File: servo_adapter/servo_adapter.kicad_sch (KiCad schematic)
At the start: 20 parts, among them J1 T4140012081-000, J2 Conn_01x10_Socket, J3 Conn_01x02_Socket, J4 T4141012051-000, U1 MUN5233T1G, U2 MUN5233T1G, U3 MUN5233T1G, U4 MUN5233T1G

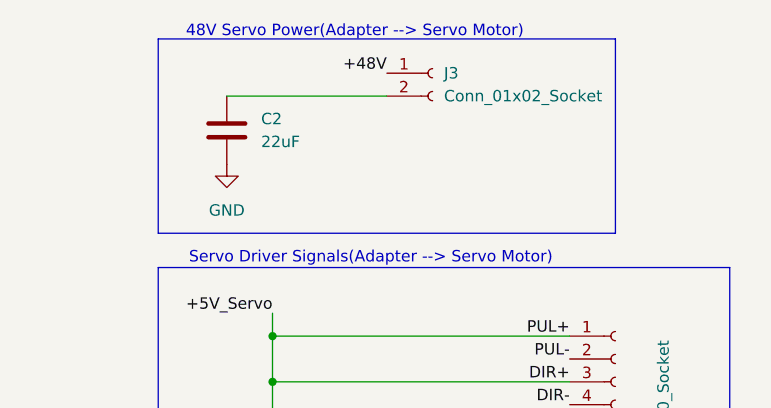
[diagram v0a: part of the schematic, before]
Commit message: Added the 2pin power connector to servo adapter board and schematic.
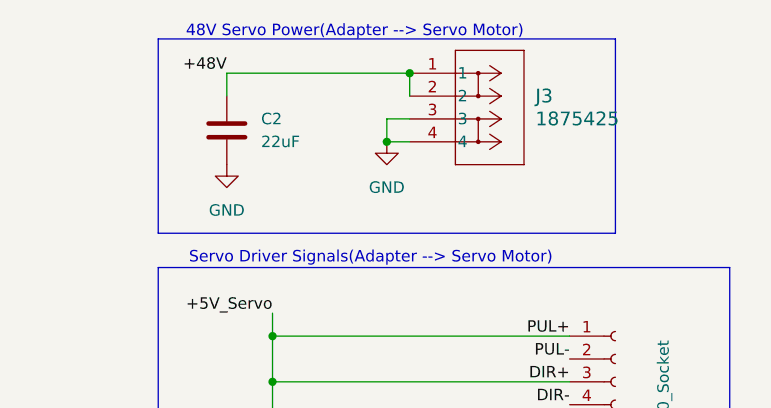
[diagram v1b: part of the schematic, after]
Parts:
- removed J3: Conn_01x02_Socket, Connector_Phoenix_MC:PhoenixContact_MCV_1,5_2-GF-3.81_1x02_P3.81mm_Vertical_ThreadedFlange_MountHole, symbol Connector:Conn_01x02_Socket
- added J3: 1875425, servo_adapter_fp:CONN_1875425, symbol 1875425:1875425
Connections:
- net +48V: now also C2.1, J3.1, J3.2
- net GND: now also J3.3, J3.4
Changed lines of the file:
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@@
 	)
 	(junction
+		(at 241.3 29.21)
+		(diameter 0)
+		(color 0 0 0 0)
+	)
+	(junction
 		(at 241.3 86.36)
 		(diameter 0)
@@
 	)
 	(junction
+		(at 243.84 21.59)
+		(diameter 0)
+		(color 0 0 0 0)
+	)
+	(junction
 		(at 33.02 38.1)
 		(diameter 0)
@@
 	(wire
 		(pts
+			(xy 223.52 21.59) (xy 223.52 24.13)
+		)
+		(stroke
+			(width 0)
+			(type default)
+		)
+	)
+	(wire
+		(pts
 			(xy 228.6 50.8) (xy 228.6 48.26)
 		)
@@
 	(wire
 		(pts
+			(xy 241.3 26.67) (xy 241.3 29.21)
+		)
+		(stroke
+			(width 0)
+			(type default)
+		)
+	)
+	(wire
+		(pts
 			(xy 81.28 165.1) (xy 81.28 170.18)
 		)
@@
 	(wire
 		(pts
+			(xy 243.84 29.21) (xy 241.3 29.21)
+		)
+		(stroke
+			(width 0)
+			(type default)
+		)
+	)
+	(wire
+		(pts
 			(xy 228.6 78.74) (xy 228.6 86.36)
 		)
@@
 	(wire
 		(pts
+			(xy 223.52 21.59) (xy 243.84 21.59)
+		)
+		(stroke
+			(width 0)
+			(type default)
+		)
+	)
+	(wire
+		(pts
+			(xy 243.84 26.67) (xy 241.3 26.67)
+		)
+		(stroke
+			(width 0)
+			(type default)
+		)
+	)
+	(wire
+		(pts
 			(xy 25.4 30.48) (xy 38.1 30.48)
 		)
@@
 	(wire
 		(pts
-			(xy 38.1 35.56) (xy 33.02 35.56)
+			(xy 243.84 21.59) (xy 243.84 24.13)
 		)
 		(stroke
@@
 	(wire
 		(pts
-			(xy 261.62 71.12) (xy 228.6 71.12)
+			(xy 38.1 35.56) (xy 33.02 35.56)
 		)
 		(stroke
@@
 	(wire
 		(pts
-			(xy 38.1 38.1) (xy 33.02 38.1)
+			(xy 261.62 71.12) (xy 228.6 71.12)
 		)
 		(stroke
@@
 	(wire
 		(pts
-			(xy 30.48 78.74) (xy 46.99 78.74)
+			(xy 38.1 38.1) (xy 33.02 38.1)
 		)
 		(stroke
@@
 	(wire
 		(pts
-			(xy 223.52 24.13) (xy 241.3 24.13)
+			(xy 30.48 78.74) (xy 46.99 78.74)
 		)
 		(stroke
@@
 	)
 	(label "+48V"
-		(at 241.3 21.59 180)
+		(at 223.52 21.59 180)
 		(effects
 			(font
@@
 	)
 	(symbol
+		(lib_id "power:GND")
+		(at 241.3 29.21 0)
+		(unit 1)
+		(exclude_from_sim no)
+		(in_bom yes)
+		(on_board yes)
+		(dnp no)
+		(fields_autoplaced yes)
+		(property "Reference" "#PWR011"
+			(at 241.3 35.56 0)
+			(effects
+				(font
+					(size 1.27 1.27)
+				)
+				(hide yes)
+			)
+		)
+		(property "Value" "GND"
+			(at 241.3 34.29 0)
+			(effects
+				(font
+					(size 1.27 1.27)
+				)
+			)
+		)
+		(property "Footprint" ""
+			(at 241.3 29.21 0)
+			(effects
+				(font
+					(size 1.27 1.27)
+				)
+				(hide yes)
+			)
+		)
+		(property "Datasheet" ""
+			(at 241.3 29.21 0)
+			(effects
+				(font
+					(size 1.27 1.27)
+				)
+				(hide yes)
+			)
+		)
+		(property "Description" "Power symbol creates a global label with name \"GND\" , ground"
+			(at 241.3 29.21 0)
+			(effects
+				(font
+					(size 1.27 1.27)
+				)
+				(hide yes)
+			)
+		)
+		(pin "1"
+		)
+		(instances
+			(project "servo_adapter"
+				(path "/d2a6932a-1682-4170-bbbb-2fb2c0f935d7"
+					(reference "#PWR011")
+					(unit 1)
+				)
+			)
+		)
+	)
+	(symbol
 		(lib_id "Device:C")
 		(at 223.52 27.94 0)
@@
 	)
 	(symbol
-		(lib_id "Connector:Conn_01x02_Socket")
-		(at 246.38 21.59 0)
-		(unit 1)
-		(exclude_from_sim no)
-		(in_bom yes)
-		(on_board yes)
-		(dnp no)
-		(fields_autoplaced yes)
-		(property "Reference" "J3"
-			(at 247.65 21.5899 0)
-			(effects
-				(font
-					(size 1.27 1.27)
-				)
-				(justify left)
-			)
-		)
-		(property "Value" "Conn_01x02_Socket"
-			(at 247.65 24.1299 0)
-			(effects
-				(font
-					(size 1.27 1.27)
-				)
-				(justify left)
-			)
-		)
-		(property "Footprint" "Connector_Phoenix_MC:PhoenixContact_MCV_1,5_2-GF-3.81_1x02_P3.81mm_Vertical_ThreadedFlange_MountHole"
-			(at 246.38 21.59 0)
-			(effects
-				(font
-					(size 1.27 1.27)
-				)
-				(hide yes)
-			)
-		)
-		(property "Datasheet" "~"
-			(at 246.38 21.59 0)
-			(effects
-				(font
-					(size 1.27 1.27)
-				)
-				(hide yes)
-			)
-		)
-		(property "Description" "Generic connector, single row, 01x02, script generated"
-			(at 246.38 21.59 0)
-			(effects
-				(font
-					(size 1.27 1.27)
-				)
-				(hide yes)
-			)
-		)
-		(pin "2"
-		)
-		(pin "1"
-		)
-		(instances
-			(project ""
-				(path "/d2a6932a-1682-4170-bbbb-2fb2c0f935d7"
-					(reference "J3")
-					(unit 1)
-				)
-			)
-		)
-	)
-	(symbol
 		(lib_id "power:PWR_FLAG")
 		(at 54.61 72.39 180)
@@
 					(unit 1)
 				)
+			)
+		)
+	)
+	(symbol
+		(lib_id "1875425:1875425")
+		(at 243.84 21.59 0)
+		(unit 1)
+		(exclude_from_sim no)
+		(in_bom yes)
+		(on_board yes)
+		(dnp no)
+		(fields_autoplaced yes)
+		(property "Reference" "J3"
+			(at 257.81 24.1299 0)
+			(effects
+				(font
+					(size 1.524 1.524)
+				)
+				(justify left)
+			)
+		)
+		(property "Value" "1875425"
+			(at 257.81 26.6699 0)
+			(effects
+				(font
+					(size 1.524 1.524)
+				)
+				(justify left)
+			)
+		)
+		(property "Footprint" "servo_adapter_fp:CONN_1875425"
+			(at 243.84 21.59 0)
+			(effects
+				(font
+					(size 1.27 1.27)
+					(italic yes)
+				)
+				(hide yes)
+			)
+		)
+		(property "Datasheet" "1875425"
+			(at 243.84 21.59 0)
+			(effects
+				(font
+					(size 1.27 1.27)
+					(italic yes)
+				)
+				(hide yes)
+			)
+		)
+		(property "Description" ""
+			(at 243.84 21.59 0)
+			(effects
+				(font
+					(size 1.27 1.27)
+				)
+				(hide yes)
+			)
+		)
+		(pin "3"
+		)
+		(pin "2"
+		)
+		(pin "4"
+		)
+		(pin "1"
+		)
+		(instances
+			(project ""
+				(path "/d2a6932a-1682-4170-bbbb-2fb2c0f935d7"
+					(reference "J3")
+					(unit 1)
+				)
